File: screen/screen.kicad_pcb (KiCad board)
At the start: 4 copper layers, 41.9 x 30 mm, 34 parts, among them J1 USB_C_Receptacle_USB2.0, J2 Conn_01x02_Female, J3 Conn_01x12_Female, J4 Conn_01x06_Female, SW1 SW_DPDT_x2, SW2 SW_Push, SW3 SW_Push, U1 TP4056_[C16581], U3 SPX3819M5-L-3-3, U4 ESP-12E

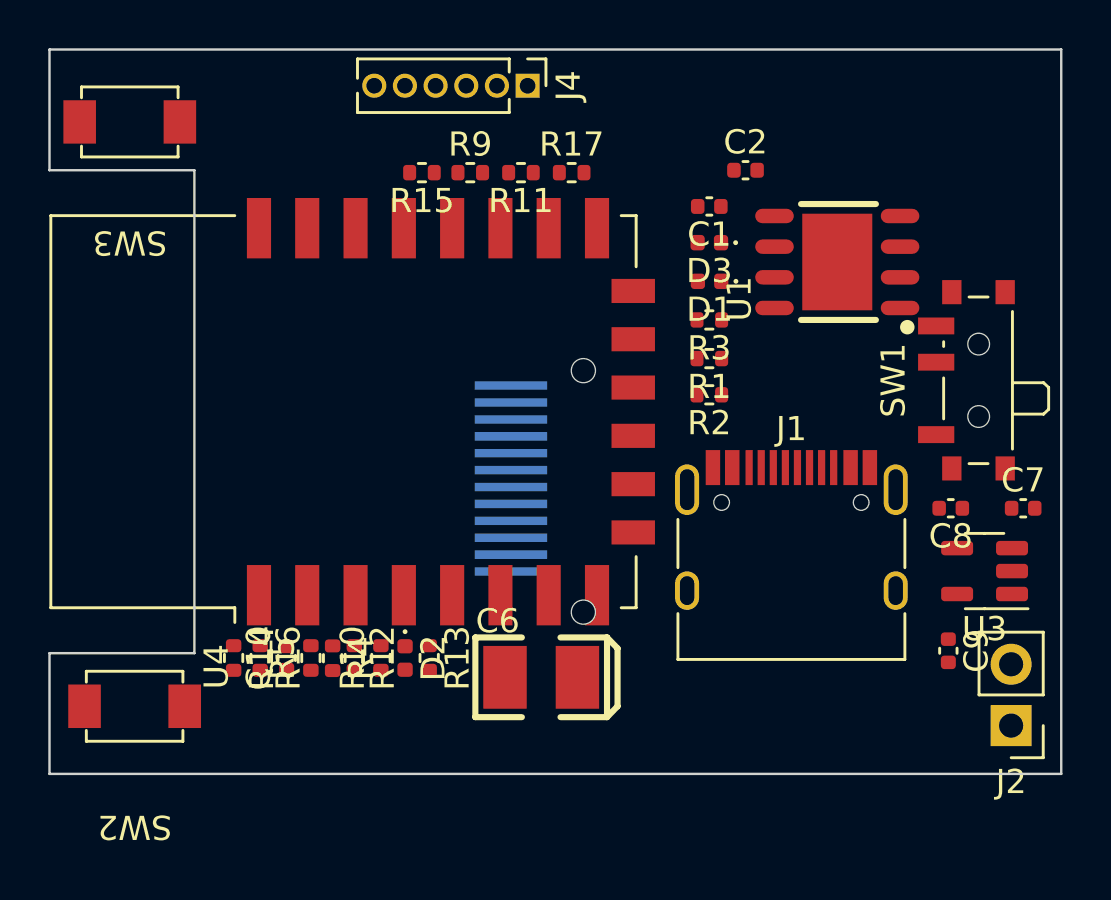
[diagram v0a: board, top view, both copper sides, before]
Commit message: screen finish
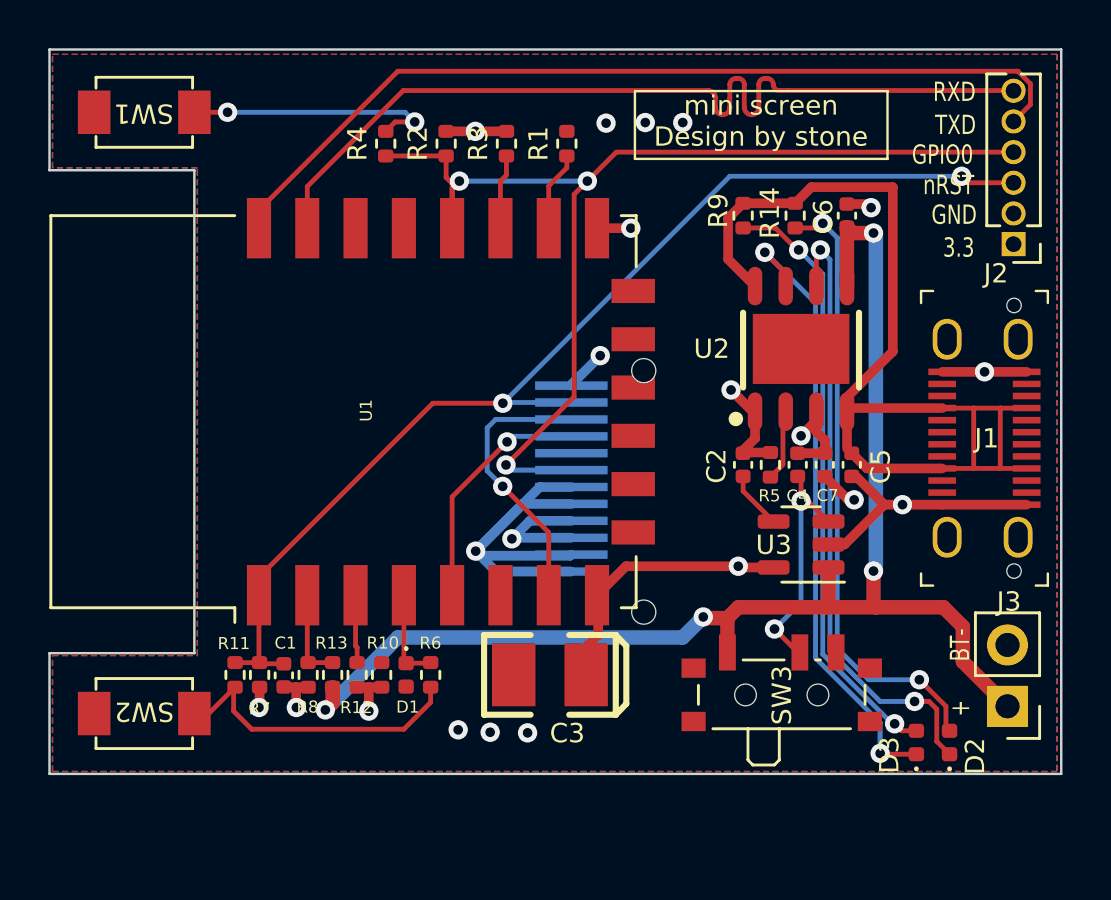
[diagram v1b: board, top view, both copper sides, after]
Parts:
- J1: footprint Connector_USB:USB_C_Receptacle_HRO_TYPE-C-31-M-12 -> digikey-footprints:USB-C_Female_Vert_DX07S024WJ3R400
- moved D2 23.0 mm to (146.2, 113.4), turned to 90 degrees
- moved J2 21.2 mm to (148.9, 92.8), turned to 180 degrees
- moved D3 20.9 mm to (144.9, 113.4), turned to 90 degrees
- moved SW3 14.9 mm to (139.3, 111.1), turned to 0 degrees
- moved C5 13.0 mm to (142.2, 101.9), turned to 90 degrees
- moved J1 10.6 mm to (148.9, 100.8), turned to -90 degrees
- moved C4 9.51 mm to (140.0, 101.9), turned to 90 degrees
- moved C7 9.25 mm to (141.1, 101.9), turned to 90 degrees
- moved C2 8.79 mm to (137.7, 101.9), turned to 90 degrees
- moved U3 7.68 mm to (140.1, 105.2)
- moved R9 7.55 mm to (137.7, 91.6), turned to 90 degrees
- moved R14 6.91 mm to (139.9, 91.6), turned to 90 degrees
- moved R5 6.51 mm to (138.8, 101.9), turned to 90 degrees
- moved C6 5.71 mm to (142.0, 91.6), turned to 90 degrees
- moved U2 3.90 mm to (140.1, 97.1), turned to 0 degrees
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- renumbered C10 to C1, C8 to C2, C6 to C3, C7 to C4, C2 to C5, C1 to C6, C9 to C7, D2 to D1, D3 to D2, D1 to D3, J4 to J2, J2 to J3, J3 to J4, R17 to R1, R14 to R11, R4 to R13, R1 to R14, R9 to R2, R11 to R3, R15 to R4, R3 to R5, R13 to R6, R16 to R7, R5 to R8, R2 to R9, SW3 to SW1, SW1 to SW3, U4 to U1, U1 to U2
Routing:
- net +BATT: track 0.00 -> 56.0 mm, vias 0 -> 4
- net /GPIO0: track 0.00 -> 47.1 mm, vias 0 -> 3
- net GND: track 0.00 -> 47.0 mm, vias 0 -> 15
- net /nRST: track 0.00 -> 46.7 mm, vias 0 -> 2
- net Net-(C2-Pad2): track 0.00 -> 42.2 mm
- net /RXD: track 0.00 -> 37.3 mm
- net /TXD: track 0.00 -> 37.1 mm
- net Net-(D1-Pad1): track 0.00 -> 26.0 mm, vias 0 -> 2
- net Net-(D3-Pad1): track 0.00 -> 25.9 mm, vias 0 -> 2
- net Net-(D3-Pad2): track 0.00 -> 25.6 mm, vias 0 -> 2
- net Net-(D1-Pad2): track 0.00 -> 25.0 mm, vias 0 -> 2
- net +3V3: track 0.00 -> 23.6 mm, vias 0 -> 6
- net Net-(R13-Pad2): track 0.00 -> 12.7 mm
- net /GPIO13: track 0.00 -> 11.6 mm, vias 0 -> 1
- net Net-(R15-Pad2): track 0.00 -> 10.7 mm, vias 0 -> 2
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- added copper zone on In2.Cu, net +3V3
- added copper zone on B.Cu, net GND
- added copper zone on F.Cu, net GND
- added copper zone on In1.Cu, net GND
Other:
- board text added: "+"
- board text added: "3.3"
- board text added: "BT-"
- board text added: "GND"
- board text added: "GPIO0"
- board text added: "RXD"
- board text added: "Release my personality and pursuing my dream."
- board text added: "TXD"
- board text added: "mini screen Design by stone"
- board text added: "nRST"
